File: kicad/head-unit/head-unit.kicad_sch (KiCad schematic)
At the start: 8 parts, among them J1 Raspberry Pi, J2 DAC Connector, J3 Programmer Port, J4 Steering Wheel, SW1 SW RST, SW2 SW Mute, U1 STM32L151C6TxA

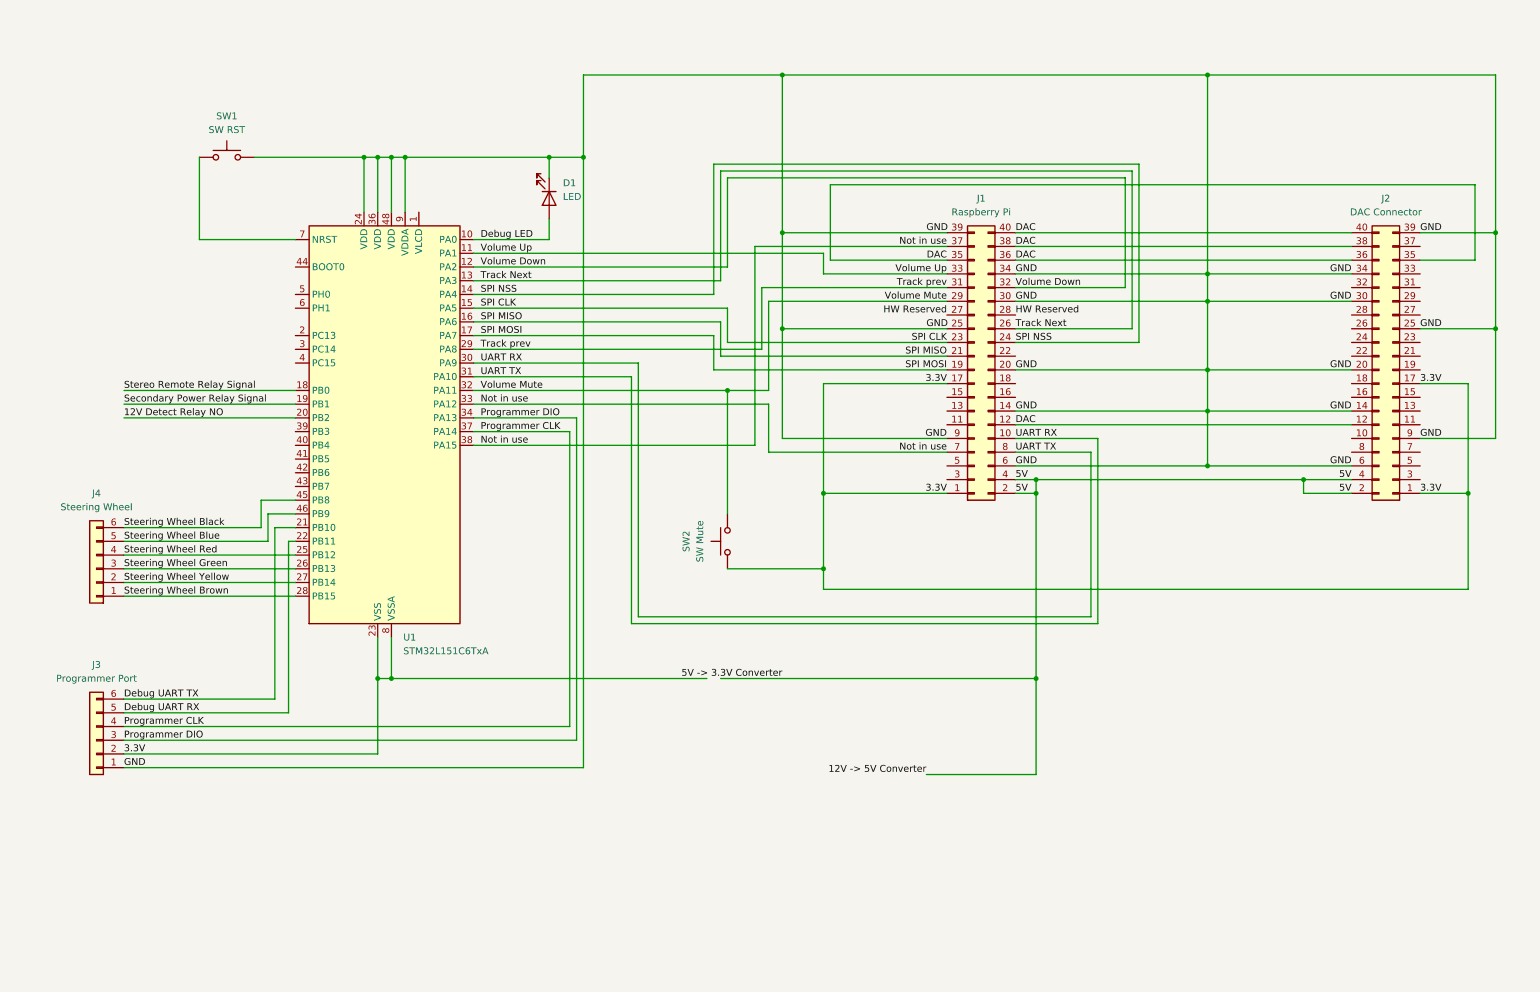
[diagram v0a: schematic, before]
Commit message: Relays, cleanup
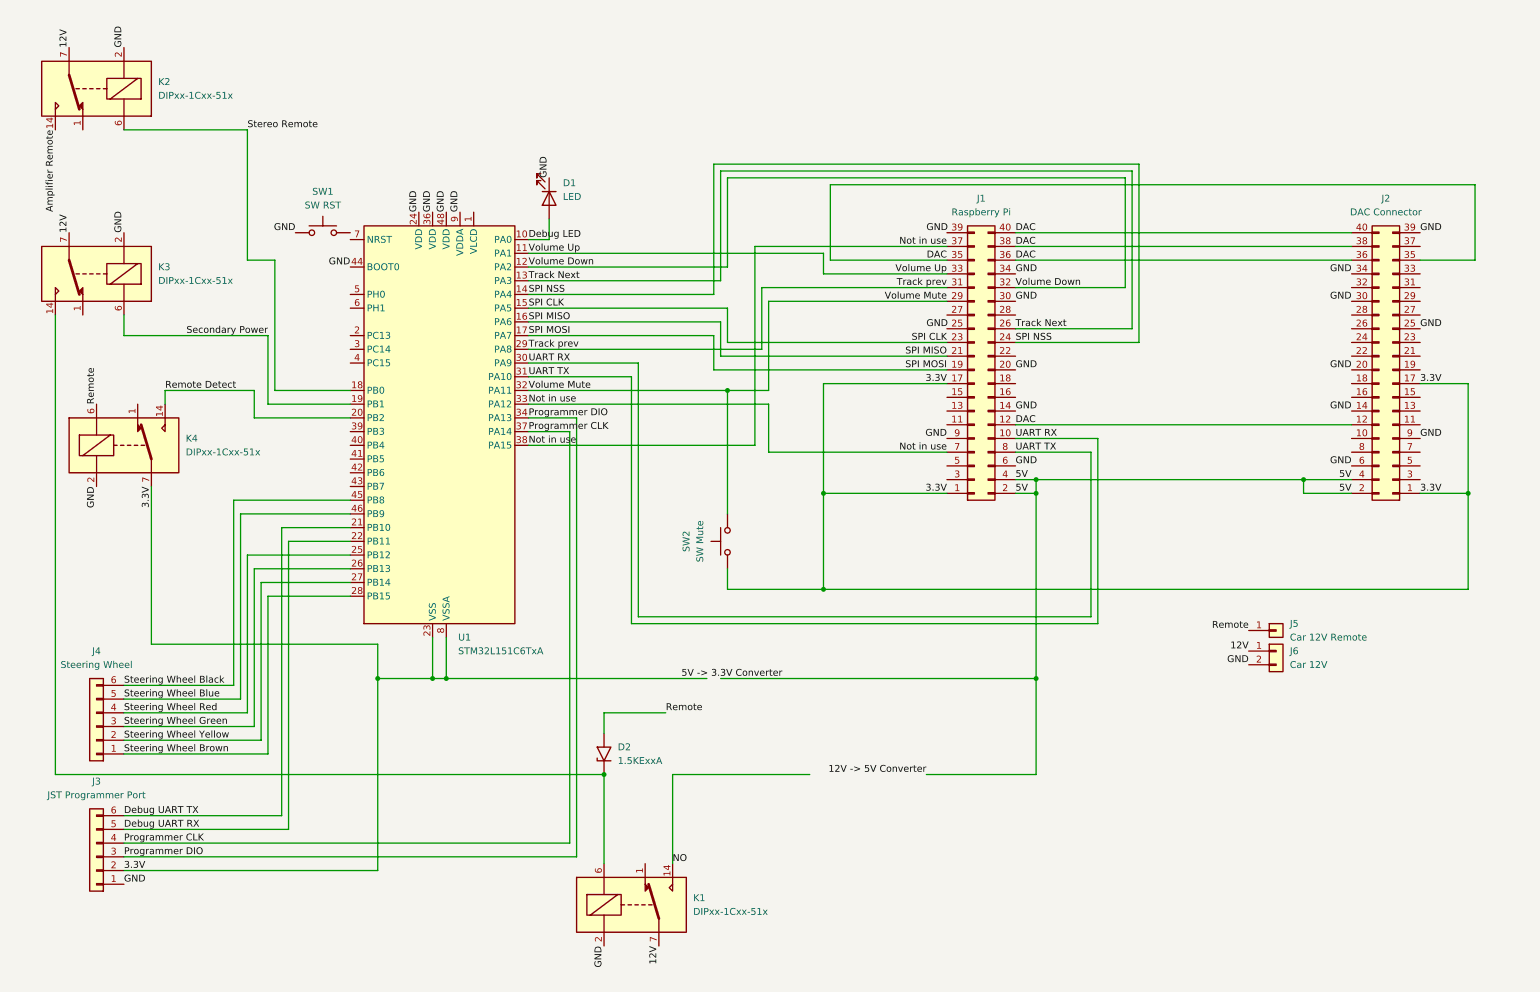
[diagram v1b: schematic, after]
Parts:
- added D2: 1.5KExxA, Diode_THT:D_DO-201AE_P15.24mm_Horizontal, symbol Diode:1.5KExxA
- added J5: Car 12V Remote, symbol Connector_Generic:Conn_01x01
- added J6: Car 12V, symbol Connector_Generic:Conn_01x02
- added K1, K2, K3, K4: DIPxx-1Cxx-51x, Relay_THT:Relay_StandexMeder_DIP_LowProfile, symbol Relay:DIPxx-1Cxx-51x
- J3: value Programmer Port -> JST Programmer Port
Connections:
- net 3.3V: now also K4.7, K4.8
- net GND: now also SW1.1, U1.44 (BOOT0), J6.2 (Pin_2), K1.2, K2.2, K3.2, K4.2; no longer J1.25 (Pin_25), J1.39 (Pin_39), SW1.2
- net at U1.7 (NRST): no longer SW1.1
- net 12V Detect Relay NO renamed Remote Detect
- net Remote Detect: now also K4.14
- net HW Reserved: no longer names the net of J1.27 (Pin_27)
- net HW Reserved: no longer J1.28 (Pin_28)
- net Secondary Power Relay Signal renamed Secondary Power
- net Secondary Power: now also K3.6
- net Stereo Remote Relay Signal renamed Stereo Remote
- net Stereo Remote: now also K2.6
- new net: D2.1 (A1), K1.6, K3.14
- new net 12V: J6.1 (Pin_1), K1.7, K1.8, K2.7, K2.8, K3.7, K3.8
- new net Amplifier Remote: K2.14
- new net NO: K1.14
- new net Remote: D2.2 (A2), J5.1 (Pin_1), K4.6
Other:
- moved on the sheet: J3, J4, SW1, U1

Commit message: Work on head unit
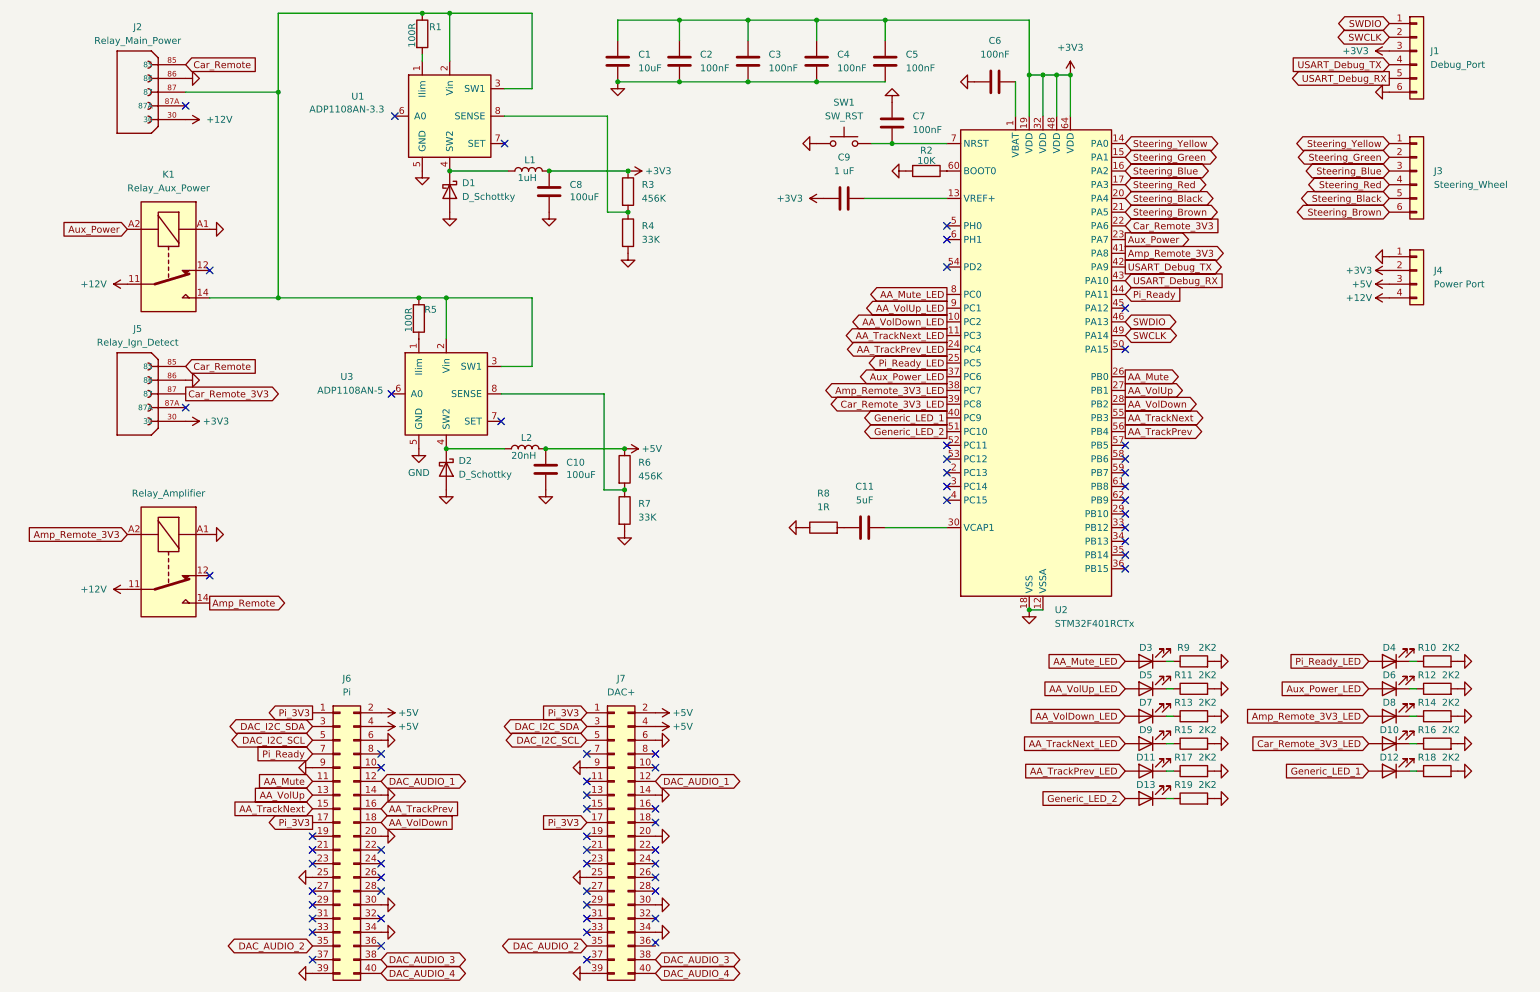
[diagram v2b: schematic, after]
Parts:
- removed D1: LED, symbol Device:LED
- removed D2: 1.5KExxA, Diode_THT:D_DO-201AE_P15.24mm_Horizontal, symbol Diode:1.5KExxA
- removed J1: Raspberry Pi, symbol Connector_Generic:Conn_02x20_Odd_Even
- removed J2: DAC Connector, symbol Connector_Generic:Conn_02x20_Odd_Even
- removed J4: Steering Wheel, symbol Connector_Generic:Conn_01x06
- removed J5: Car 12V Remote, symbol Connector_Generic:Conn_01x01
- removed J6: Car 12V, symbol Connector_Generic:Conn_01x02
- removed K1, K2, K3, K4: DIPxx-1Cxx-51x, Relay_THT:Relay_StandexMeder_DIP_LowProfile, symbol Relay:DIPxx-1Cxx-51x
- removed SW2: SW Mute, symbol Switch:SW_Push
- removed U1: STM32L151C6TxA, Package_QFP:LQFP-48_7x7mm_P0.5mm, symbol MCU_ST_STM32L1:STM32L151C6TxA
- added C1: 10uF, Capacitor_SMD:C_0201_0603Metric, symbol Device:C
- added C10: 100uF, Capacitor_SMD:C_1206_3216Metric, symbol Device:C
- added C11: 5uF, Capacitor_SMD:C_0603_1608Metric, symbol Device:C
- added C2, C3, C4, C5, C6, C7: 100nF, Capacitor_SMD:C_0402_1005Metric, symbol Device:C
- added C8: 100uF, Capacitor_SMD:C_0402_1005Metric, symbol Device:C
- added C9: 1 uF, Capacitor_SMD:C_0402_1005Metric, symbol Device:C
- added D1, D2: D_Schottky, Diode_SMD:D_0603_1608Metric, symbol Device:D_Schottky
- added D10, D11, D12, D13, D3, D4, D5, D6, D7, D8, D9: LED, LED_SMD:LED_0603_1608Metric, symbol Device:LED
- added J1: Debug_Port, Connector_PinHeader_2.54mm:PinHeader_1x06_P2.54mm_Vertical, symbol Connector_Generic:Conn_01x06
- added J2: Relay_Main_Power, VCF4-1000:TE_VCF4-1000, symbol VCF4-1000:VCF4-1000
- added J4: Power Port, Connector_PinHeader_2.54mm:PinHeader_1x04_P2.54mm_Vertical, symbol Connector_Generic:Conn_01x04
- added J5: Relay_Ign_Detect, VCF4-1000:TE_VCF4-1000, symbol VCF4-1000:VCF4-1000
- added J6: Pi, Connector_PinHeader_2.54mm:PinHeader_2x20_P2.54mm_Vertical, symbol Connector_Generic:Conn_02x20_Odd_Even
- added J7: DAC+, Connector_PinHeader_2.54mm:PinHeader_2x20_P2.54mm_Vertical, symbol Connector_Generic:Conn_02x20_Odd_Even
- added K1: Relay_Aux_Power, Relay_THT:Relay_SPDT_Finder_36.11, symbol Relay:Relay_SPDT
- added K2: Relay_Amplifier, Relay_THT:Relay_SPDT_Finder_36.11, symbol Relay:Relay_SPDT
- added L1: 1uH, Inductor_SMD:L_0402_1005Metric, symbol Device:L
- added L2: 20nH, Inductor_SMD:L_0603_1608Metric, symbol Device:L
- added R1, R5: 100R, Resistor_SMD:R_0402_1005Metric, symbol Device:R
- added R10, R11, R12, R13, R14, R15, R16, R17, R18, R19, R9: 2K2, Resistor_SMD:R_0402_1005Metric, symbol Device:R
- added R2: 10K, Resistor_SMD:R_0402_1005Metric, symbol Device:R
- added R3, R6: 456K, Resistor_SMD:R_0402_1005Metric, symbol Device:R
- added R4, R7: 33K, Resistor_SMD:R_0402_1005Metric, symbol Device:R
- added R8: 1R, Resistor_SMD:R_0402_1005Metric, symbol Device:R
- added U1: ADP1108AN-3.3, Package_DIP:DIP-8_W7.62mm, symbol Regulator_Switching:ADP1108AN-3.3
- added U2: STM32F401RCTx, Package_QFP:LQFP-64_10x10mm_P0.5mm, symbol MCU_ST_STM32F4:STM32F401RCTx
- added U3: ADP1108AN-5, Package_DIP:DIP-8_W7.62mm, symbol Regulator_Switching:ADP1108AN-5
- J3: value JST Programmer Port -> Steering_Wheel; footprint (none) -> Connector_PinHeader_2.54mm:PinHeader_1x06_P2.54mm_Vertical
- SW1: value SW RST -> SW_RST; footprint (none) -> Button_Switch_SMD:SW_Push_1P1T_NO_CK_KSC7xxJ
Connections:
- net GND: now also C1.2, C10.2, C2.2, C3.2, C4.2, C5.2, C6.1, C7.1, C8.2, D1.2 (A), D2.2 (A), J1.6 (Pin_6), J2.86, J4.1 (Pin_1), J5.86, J6.14 (Pin_14), J6.20 (Pin_20), J6.25 (Pin_25), J6.30 (Pin_30), J6.34 (Pin_34), J6.39 (Pin_39), J6.6 (Pin_6), J6.9 (Pin_9), J7.14 (Pin_14), J7.20 (Pin_20), J7.25 (Pin_25), J7.30 (Pin_30), J7.34 (Pin_34), J7.39 (Pin_39), J7.6 (Pin_6), J7.9 (Pin_9), K1.A1, K2.A1, R10.2, R11.2, R12.2, R13.2, R14.2, R15.2, R16.2, R17.2, R18.2, R19.2, R2.2, R4.2, R7.2, R8.1, R9.2, U1.5 (GND), U2.12 (VSSA), U2.18 (VSS), U2.31 (VSS), U2.47 (VSS), U2.63 (VSS), U3.5 (GND); no longer J3.1 (Pin_1)
- net at SW1.2: now also C7.2, U2.7 (NRST)
- net 3.3V renamed Steering_Green
- net Steering_Green: now also U2.15 (PA1)
- net Debug UART RX renamed Steering_Black
- net Steering_Black: now also U2.20 (PA4)
- net Debug UART TX renamed Steering_Brown
- net Steering_Brown: now also U2.21 (PA5)
- net Programmer CLK renamed Steering_Red
- net Steering_Red: now also U2.17 (PA3)
- net Programmer DIO renamed Steering_Blue
- net Steering_Blue: now also U2.16 (PA2)
- new net: D5.1 (K), R11.1
- new net: C6.2, U2.1 (VBAT)
- new net: C11.2, R8.2
- new net: D11.1 (K), R17.1
- new net: D2.1 (K), L2.1, U3.4 (SW2)
- new net: C9.1, U2.13 (VREF+)
- new net: C11.1, U2.30 (VCAP1)
- new net: R2.1, U2.60 (BOOT0)
- new net: D6.1 (K), R12.1
- new net: D7.1 (K), R13.1
- new net: J2.87, K1.14, R1.1, R5.1, U1.2 (Vin), U1.3 (SW1), U3.2 (Vin), U3.3 (SW1)
- new net: R1.2, U1.1 (Ilim)
- new net: R5.2, U3.1 (Ilim)
- new net: D8.1 (K), R14.1
- new net: D9.1 (K), R15.1
- new net: D1.1 (K), L1.1, U1.4 (SW2)
- new net: R3.2, R4.1, U1.8 (SENSE)
- new net: R6.2, R7.1, U3.8 (SENSE)
- new net: D13.1 (K), R19.1
- new net: D4.1 (K), R10.1
- new net: D3.1 (K), R9.1
- new net: D12.1 (K), R18.1
- new net: D10.1 (K), R16.1
- new net +12V: J2.30, J4.4 (Pin_4), K1.11, K2.11
- new net +3V3: C1.1, C2.1, C3.1, C4.1, C5.1, C8.1, C9.2, J1.3 (Pin_3), J4.2 (Pin_2), J5.30, L1.2, R3.1, U2.19 (VDD), U2.32 (VDD), U2.48 (VDD), U2.64 (VDD)
- new net +5V: C10.1, J4.3 (Pin_3), J6.2 (Pin_2), J6.4 (Pin_4), J7.2 (Pin_2), J7.4 (Pin_4), L2.2, R6.1
- new net AA_Mute: J6.11 (Pin_11), U2.26 (PB0)
- new net AA_Mute_LED: D3.2 (A), U2.8 (PC0)
- new net AA_TrackNext: J6.15 (Pin_15), U2.55 (PB3)
- new net AA_TrackNext_LED: D9.2 (A), U2.11 (PC3)
- new net AA_TrackPrev: J6.16 (Pin_16), U2.56 (PB4)
- new net AA_TrackPrev_LED: D11.2 (A), U2.24 (PC4)
- new net AA_VolDown: J6.18 (Pin_18), U2.28 (PB2)
- new net AA_VolDown_LED: D7.2 (A), U2.10 (PC2)
- new net AA_VolUp: J6.13 (Pin_13), U2.27 (PB1)
- new net AA_VolUp_LED: D5.2 (A), U2.9 (PC1)
- new net Amp_Remote: K2.14
- new net Amp_Remote_3V3: K2.A2, U2.41 (PA8)
- new net Amp_Remote_3V3_LED: D8.2 (A), U2.38 (PC7)
- new net Aux_Power: K1.A2, U2.23 (PA7)
- new net Aux_Power_LED: D6.2 (A), U2.37 (PC6)
- new net Car_Remote: J2.85, J5.85
- new net Car_Remote_3V3: J5.87, U2.22 (PA6)
- new net Car_Remote_3V3_LED: D10.2 (A), U2.39 (PC8)
- new net DAC_AUDIO_1: J6.12 (Pin_12), J7.12 (Pin_12)
- new net DAC_AUDIO_2: J6.35 (Pin_35), J7.35 (Pin_35)
- new net DAC_AUDIO_3: J6.38 (Pin_38), J7.38 (Pin_38)
- new net DAC_AUDIO_4: J6.40 (Pin_40), J7.40 (Pin_40)
- new net DAC_I2C_SCL: J6.5 (Pin_5), J7.5 (Pin_5)
- new net DAC_I2C_SDA: J6.3 (Pin_3), J7.3 (Pin_3)
- new net Generic_LED_1: D12.2 (A), U2.40 (PC9)
- new net Generic_LED_2: D13.2 (A), U2.51 (PC10)
- new net Pi_3V3: J6.1 (Pin_1), J6.17 (Pin_17), J7.1 (Pin_1), J7.17 (Pin_17)
- new net Pi_Ready: J6.7 (Pin_7), U2.44 (PA11)
- new net Pi_Ready_LED: D4.2 (A), U2.25 (PC5)
- new net SWCLK: J1.2 (Pin_2), U2.49 (PA14)
- new net SWDIO: J1.1 (Pin_1), U2.46 (PA13)
- new net Steering_Yellow: J3.1 (Pin_1), U2.14 (PA0)
- new net USART_Debug_RX: J1.5 (Pin_5), U2.43 (PA10)
- new net USART_Debug_TX: J1.4 (Pin_4), U2.42 (PA9)
- no-connect marks 0 -> 66
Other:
- title: twingo-head-unit -> (none)
